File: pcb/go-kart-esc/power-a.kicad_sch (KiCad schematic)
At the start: 6 parts, among them Q1 IRLB8721PBF, Q2 IRLB8721PBF, Q3 IRLB8721PBF, Q4 IRLB8721PBF

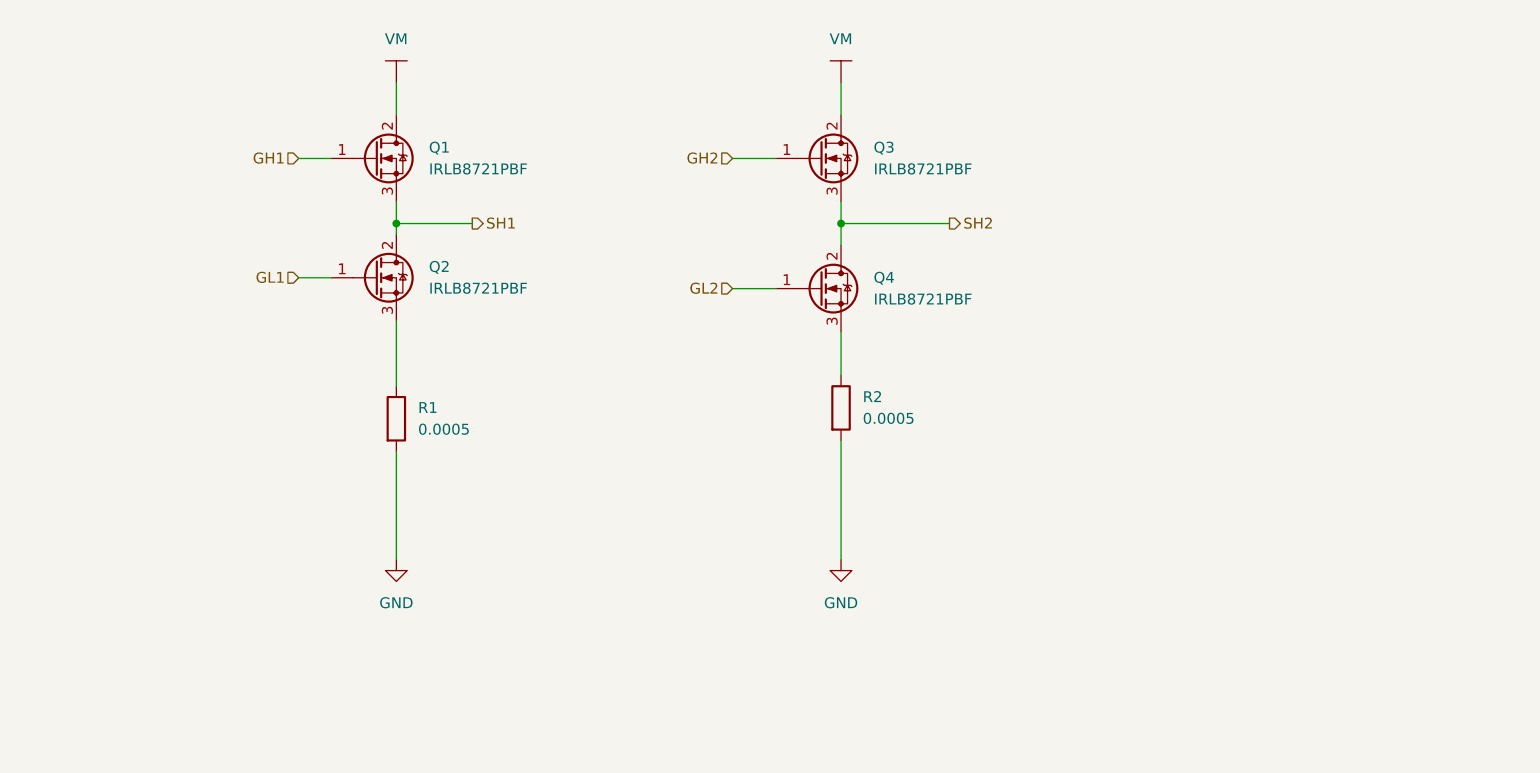
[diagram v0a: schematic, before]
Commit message: Poggers
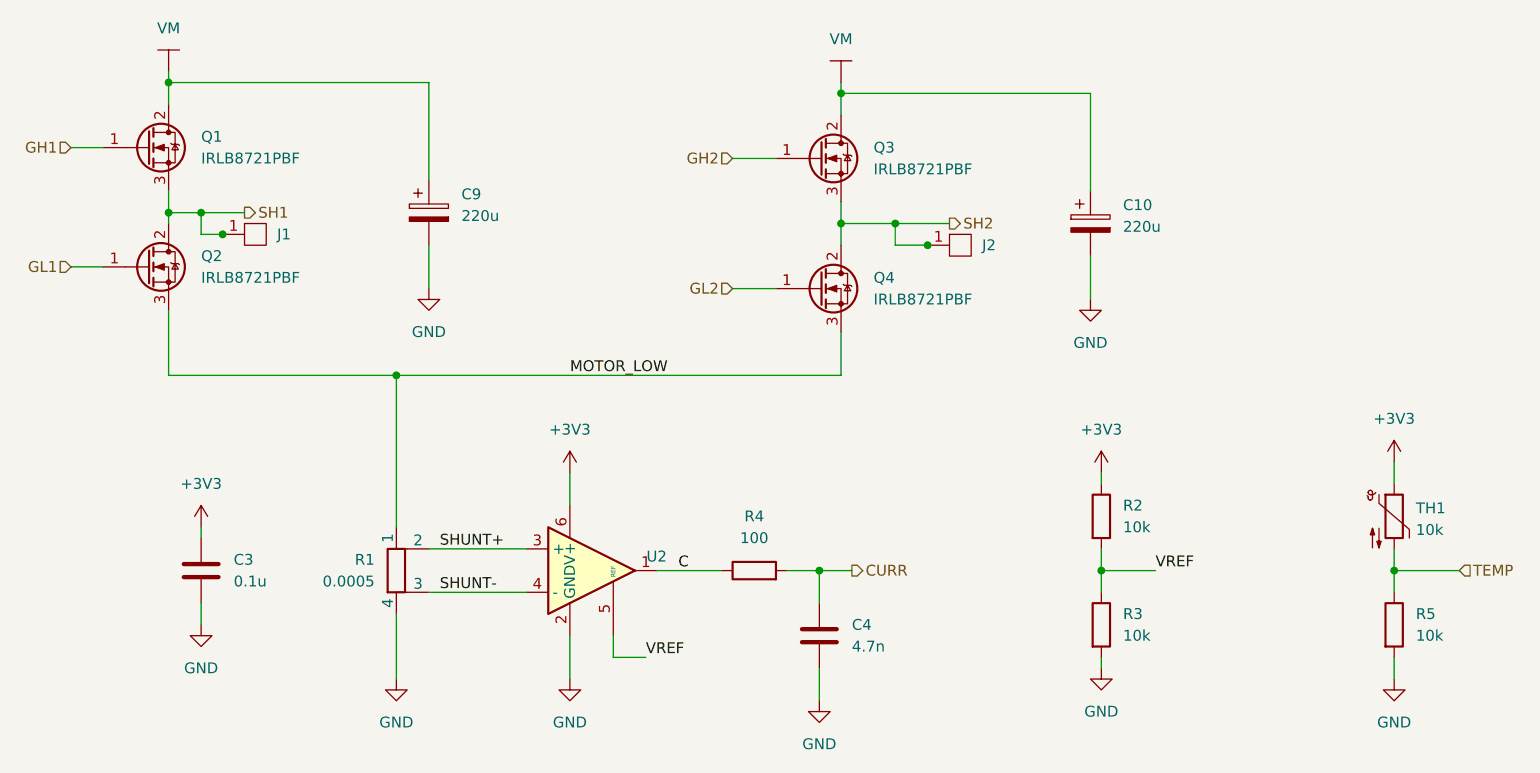
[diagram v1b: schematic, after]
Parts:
- removed R1: 0.0005, symbol Device:R
- added C10, C9: 220u, symbol Device:C_Polarized
- added C3: 0.1u, symbol Device:C
- added C4: 4.7n, symbol Device:C
- added J1, J2: ~, symbol ESC:MotorTab
- added R1: 0.0005, symbol Device:R_Shunt
- added R3, R5: 10k, symbol Device:R
- added R4: 100, symbol Device:R
- added TH1: 10k, symbol Device:Thermistor_NTC
- added U2: ~, symbol ESC:INA185
- R2: value 0.0005 -> 10k
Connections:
- net GND: now also C10.2, C3.2, C4.2, C9.2, R1.4, R3.2, R5.2, U2.2 (GND); no longer R2.2
- net SH1: now also J1.1
- net SH2: now also J2.1
- net +3V3: now reaches R2.1
- net +3V3: now also C3.1, TH1.1, U2.6 (V+); no longer Q4.3 (S)
- net MOTOR_LOW: now reaches Q2.3 (S)
- net MOTOR_LOW: now also Q4.3 (S), R1.1
- net at Q1.2 (D): now also C9.1
- net at Q3.2 (D): now also C10.1
- new net C: R4.1, U2.1
- new net CURR: C4.1, R4.2
- new net SHUNT+: R1.2, U2.3 (+)
- new net SHUNT-: R1.3, U2.4 (-)
- new net TEMP: R5.1, TH1.2
- new net VREF: R2.2, R3.1, U2.5 (REF)
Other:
- moved on the sheet: Q1, Q2

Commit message: ooga booga
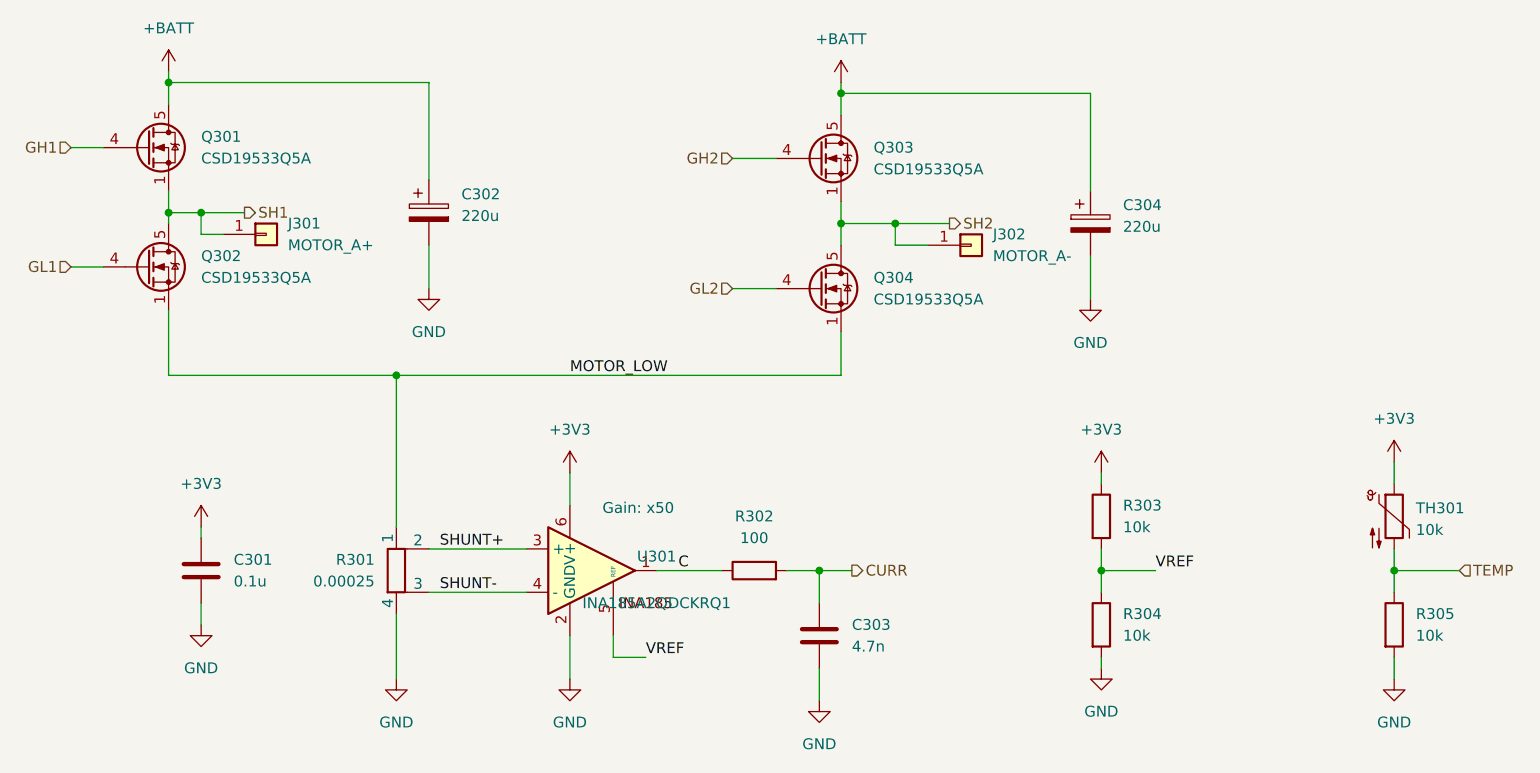
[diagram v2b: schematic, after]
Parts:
- removed J1, J2: ~, symbol ESC:MotorTab
- removed Q1, Q2, Q3, Q4: IRLB8721PBF, Package_TO_SOT_THT:TO-220-3_Vertical, symbol Transistor_FET:IRLB8721PBF
- added J301: MOTOR_A+, ESC:Motor_Solder_Pad, symbol Connector_Generic:Conn_01x01
- added J302: MOTOR_A-, ESC:Motor_Solder_Pad, symbol Connector_Generic:Conn_01x01
- added Q301, Q302, Q303, Q304: CSD19533Q5A, Package_TO_SOT_SMD:TDSON-8-1, symbol Transistor_FET:CSD19533Q5A
- C301: renamed from C3; footprint (none) -> Capacitor_SMD:C_0402_1005Metric_Pad0.74x0.62mm_HandSolder
- C302: renamed from C9; footprint (none) -> Capacitor_THT:CP_Radial_D10.0mm_P5.00mm
- C303: renamed from C4; footprint (none) -> Capacitor_SMD:C_0603_1608Metric_Pad1.08x0.95mm_HandSolder
- C304: renamed from C10; footprint (none) -> Capacitor_THT:CP_Radial_D10.0mm_P5.00mm
- R301: renamed from R1; value 0.0005 -> 0.00025; footprint (none) -> ESC:Shunt_2725
- R302: renamed from R4; footprint (none) -> Resistor_SMD:R_0402_1005Metric_Pad0.72x0.64mm_HandSolder
- R303: renamed from R2; footprint (none) -> Resistor_SMD:R_0402_1005Metric_Pad0.72x0.64mm_HandSolder
- R304: renamed from R3; footprint (none) -> Resistor_SMD:R_0402_1005Metric_Pad0.72x0.64mm_HandSolder
- R305: renamed from R5; footprint (none) -> Resistor_SMD:R_0402_1005Metric_Pad0.72x0.64mm_HandSolder
- TH301: renamed from TH1; footprint (none) -> Resistor_SMD:R_0201_0603Metric_Pad0.64x0.40mm_HandSolder
- U301: renamed from U2; value ~ -> INA185A2QDCKRQ1; footprint (none) -> Package_TO_SOT_SMD:SOT-363_SC-70-6_Handsoldering
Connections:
- net GH1: now also Q301.4 (G)
- net GH2: now also Q303.4 (G)
- net GL1: now also Q302.4 (G)
- net GL2: now also Q304.4 (G)
- net MOTOR_LOW: now also Q302.1 (S), Q302.2 (S), Q302.3 (S), Q304.1 (S), Q304.2 (S), Q304.3 (S)
- net SH1: now also J301.1 (Pin_1), Q301.1 (S), Q301.2 (S), Q301.3 (S), Q302.5 (D)
- net SH2: now also J302.1 (Pin_1), Q303.1 (S), Q303.2 (S), Q303.3 (S), Q304.5 (D)
- net +BATT: now reaches C302.1
- net +BATT: now also C304.1, Q301.5 (D), Q303.5 (D)
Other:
- note added: "Gain: x50"

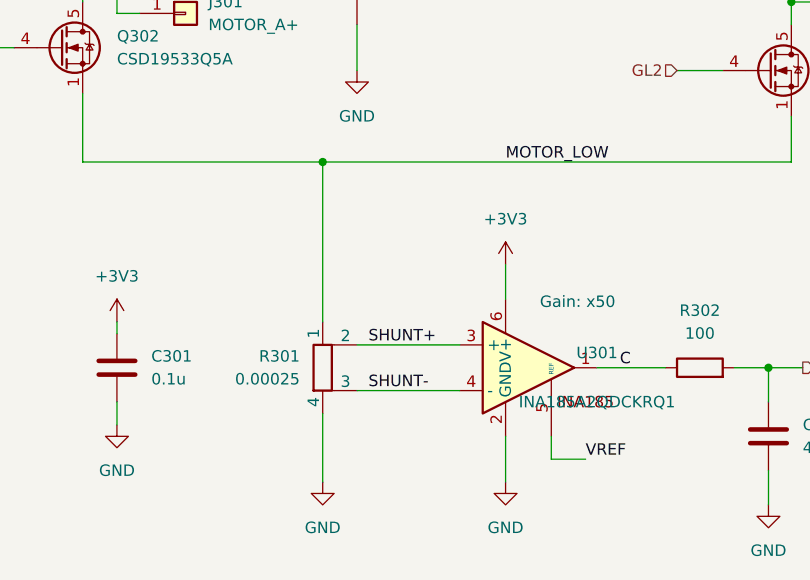
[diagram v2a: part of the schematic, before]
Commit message: ooga booga
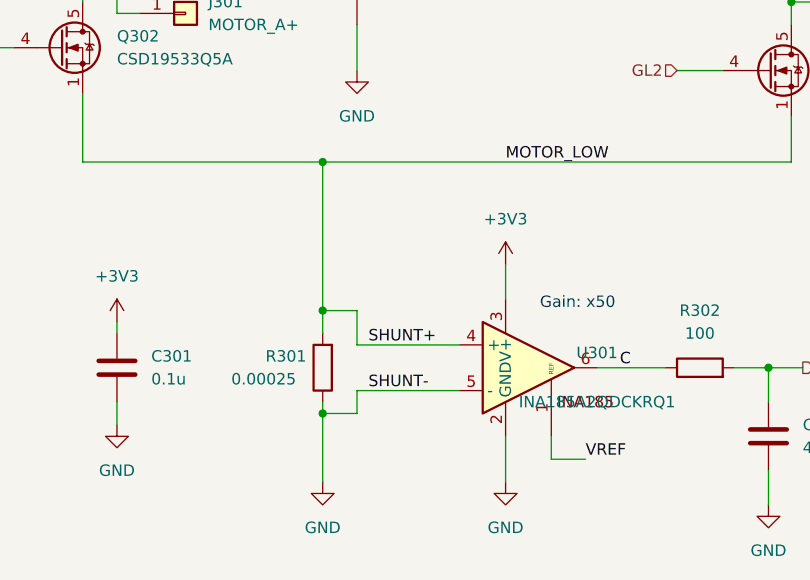
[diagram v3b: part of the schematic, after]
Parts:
- removed R301: 0.00025, ESC:Shunt_2725, symbol Device:R_Shunt
- added R301: 0.00025, ESC:Shunt_2725, symbol Device:R
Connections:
- net SHUNT+ is gone; now on net +3V3: U301.3 (V+)
- net SHUNT- is gone; now on net MOTOR_LOW: U301.4 (+)
- net +3V3: no longer U301.6 (V+)
- net C: now also U301.6; no longer U301.1
- net GND: now also U301.5 (-), R301.1
- net MOTOR_LOW: now also R301.2
- net VREF: now also U301.1 (REF); no longer U301.5 (REF)
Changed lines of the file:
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@@
   (junction (at 165.1 82.55) (diameter 0) (color 0 0 0 0)
   )
+  (junction (at 113.03 128.27) (diameter 0) (color 0 0 0 0)
+  )
   (junction (at 162.56 123.19) (diameter 0) (color 0 0 0 0)
   )
@@
   (junction (at 90.17 81.28) (diameter 0) (color 0 0 0 0)
   )
+  (junction (at 113.03 116.84) (diameter 0) (color 0 0 0 0)
+  )
   (junction (at 113.03 100.33) (diameter 0) (color 0 0 0 0)
   )
@@
     (stroke (width 0) (type default))
   )
+  (wire (pts (xy 116.84 128.27) (xy 113.03 128.27))
+    (stroke (width 0) (type default))
+  )
+  (wire (pts (xy 113.03 116.84) (xy 113.03 119.38))
+    (stroke (width 0) (type default))
+  )
+  (wire (pts (xy 116.84 116.84) (xy 113.03 116.84))
+    (stroke (width 0) (type default))
+  )
   (wire (pts (xy 138.43 130.81) (xy 138.43 133.35))
     (stroke (width 0) (type default))
   )
+  (wire (pts (xy 116.84 125.73) (xy 116.84 128.27))
+    (stroke (width 0) (type default))
+  )
   (wire (pts (xy 143.51 123.19) (xy 151.13 123.19))
     (stroke (width 0) (type default))
@@
     (stroke (width 0) (type default))
   )
+  (wire (pts (xy 116.84 120.65) (xy 116.84 116.84))
+    (stroke (width 0) (type default))
+  )
   (wire (pts (xy 152.4 90.17) (xy 157.48 90.17))
     (stroke (width 0) (type default))
   )
+  (wire (pts (xy 113.03 128.27) (xy 113.03 135.89))
+    (stroke (width 0) (type default))
+  )
   (wire (pts (xy 229.87 123.19) (xy 237.49 123.19))
     (stroke (width 0) (type default))
@@
     (stroke (width 0) (type default))
   )
-  (wire (pts (xy 113.03 128.27) (xy 113.03 135.89))
+  (wire (pts (xy 113.03 127) (xy 113.03 128.27))
     (stroke (width 0) (type default))
   )
@@
     (stroke (width 0) (type default))
   )
-  (wire (pts (xy 113.03 100.33) (xy 113.03 118.11))
+  (wire (pts (xy 113.03 100.33) (xy 113.03 116.84))
     (stroke (width 0) (type default))
   )
@@
   (symbol (lib_id "power:+BATT") (at 86.36 64.77 0) (unit 1)
     (in_bom yes) (on_board yes) (dnp no) (fields_autoplaced)
-    (property "Reference" "#PWR0609" (at 86.36 68.58 0)
+    (property "Reference" "#PWR0601" (at 86.36 68.58 0)
       (effects (font (size 1.27 1.27)) hide)
     )
@@
       (project "go-kart-esc"
         (path "/5a70b585-4866-4f79-8013-f2242aeded57/a459c41b-c6c3-40c7-8485-5a95e06155ac"
-          (reference "#PWR0609") (unit 1)
-        )
-        (path "/5a70b585-4866-4f79-8013-f2242aeded57/2f2eb473-a6d5-4b09-8c58-ce0c11f580af"
-          (reference "#PWR0309") (unit 1)
+          (reference "#PWR0601") (unit 1)
+        )
+        (path "/5a70b585-4866-4f79-8013-f2242aeded57/2f2eb473-a6d5-4b09-8c58-ce0c11f580af"
+          (reference "#PWR0301") (unit 1)
         )
       )
@@
   (symbol (lib_id "power:+BATT") (at 165.1 66.04 0) (unit 1)
     (in_bom yes) (on_board yes) (dnp no) (fields_autoplaced)
-    (property "Reference" "#PWR0601" (at 165.1 69.85 0)
+    (property "Reference" "#PWR0609" (at 165.1 69.85 0)
       (effects (font (size 1.27 1.27)) hide)
     )
@@
       (project "go-kart-esc"
         (path "/5a70b585-4866-4f79-8013-f2242aeded57/a459c41b-c6c3-40c7-8485-5a95e06155ac"
-          (reference "#PWR0601") (unit 1)
-        )
-        (path "/5a70b585-4866-4f79-8013-f2242aeded57/2f2eb473-a6d5-4b09-8c58-ce0c11f580af"
-          (reference "#PWR0301") (unit 1)
+          (reference "#PWR0609") (unit 1)
+        )
+        (path "/5a70b585-4866-4f79-8013-f2242aeded57/2f2eb473-a6d5-4b09-8c58-ce0c11f580af"
+          (reference "#PWR0309") (unit 1)
         )
       )
@@
     )
   )
-  (symbol (lib_id "Device:R_Shunt") (at 113.03 123.19 0) (unit 1)
-    (in_bom yes) (on_board yes) (dnp no) (fields_autoplaced)
-    (property "Reference" "R301" (at 110.49 121.92 0)
-      (effects (font (size 1.27 1.27)) (justify right))
-    )
-    (property "Value" "0.00025" (at 110.49 124.46 0)
-      (effects (font (size 1.27 1.27)) (justify right))
-    )
-    (property "Footprint" "ESC:Shunt_2725" (at 111.252 123.19 90)
-      (effects (font (size 1.27 1.27)) hide)
-    )
-    (property "Datasheet" "~" (at 113.03 123.19 0)
-      (effects (font (size 1.27 1.27)) hide)
-    )
-    (pin "1")
-    (pin "2")
-    (pin "3")
-    (pin "4")
-    (instances
-      (project "go-kart-esc"
-        (path "/5a70b585-4866-4f79-8013-f2242aeded57/2f2eb473-a6d5-4b09-8c58-ce0c11f580af"
-          (reference "R301") (unit 1)
-        )
-        (path "/5a70b585-4866-4f79-8013-f2242aeded57/a459c41b-c6c3-40c7-8485-5a95e06155ac"
-          (reference "R601") (unit 1)
-        )
-      )
-    )
-  )
   (symbol (lib_id "Transistor_FET:CSD19533Q5A") (at 83.82 73.66 0) (unit 1)
     (in_bom yes) (on_board yes) (dnp no) (fields_autoplaced)
@@
         )
       )
+    )
+  )
+  (symbol (lib_id "Device:R") (at 113.03 123.19 180) (unit 1)
+    (in_bom yes) (on_board yes) (dnp no)
+    (property "Reference" "R301" (at 106.68 121.92 0)
+      (effects (font (size 1.27 1.27)) (justify right))
+    )
+    (property "Value" "0.00025" (at 102.87 124.46 0)
+      (effects (font (size 1.27 1.27)) (justify right))
+    )
+    (property "Footprint" "ESC:Shunt_2725" (at 114.808 123.19 90)
+      (effects (font (size 1.27 1.27)) hide)
+    )
+    (property "Datasheet" "~" (at 113.03 123.19 0)
+      (effects (font (size 1.27 1.27)) hide)
+    )
+    (pin "1")
+    (pin "2")
+    (instances
+      (project "go-kart-esc"
+        (path "/5a70b585-4866-4f79-8013-f2242aeded57/2f2eb473-a6d5-4b09-8c58-ce0c11f580af"
+          (reference "R301") (unit 1)
+        )
+        (path "/5a70b585-4866-4f79-8013-f2242aeded57/a459c41b-c6c3-40c7-8485-5a95e06155ac"
+          (reference "R601") (unit 1)
+        )
+      )
+      (project "simulation"
+        (path "/708b3adf-a477-436e-b5ed-8e1ccf99b3d7"
+          (reference "R3") (unit 1)
+        )
+      )

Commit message: Finished PCB
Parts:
- TH301: footprint Resistor_SMD:R_0201_0603Metric_Pad0.64x0.40mm_HandSolder -> Resistor_SMD:R_0402_1005Metric_Pad0.72x0.64mm_HandSolder
